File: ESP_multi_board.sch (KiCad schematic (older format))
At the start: 20 parts, among them P101 CONN_01X02, P102 CONN_01X06, P103 CONN_01X02, P104 CONN_01X06, P105 CONN_01X12, P106 CONN_01X03, P107 JUMPER1, P108 CONN_I2C_MPU6050, P109 CONN_01X03, P110 CONN_01X03, P111 CONN_DIGITAL, P112 CONN_I2C, U101 L293DD, U102 ESP-12, U103 MAX11605EEE+, U104 MCP23008

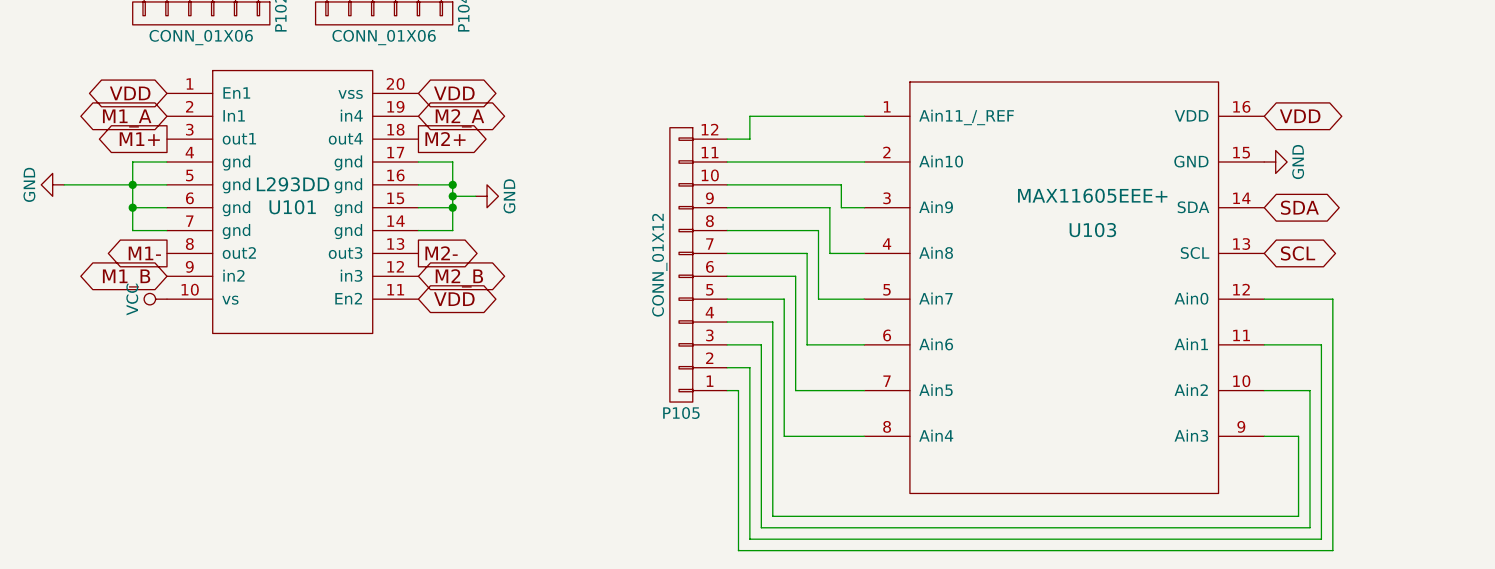
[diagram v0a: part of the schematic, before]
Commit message: pendiente de enrutar, TODO: incluir diodos baterias, meditar los jumpers
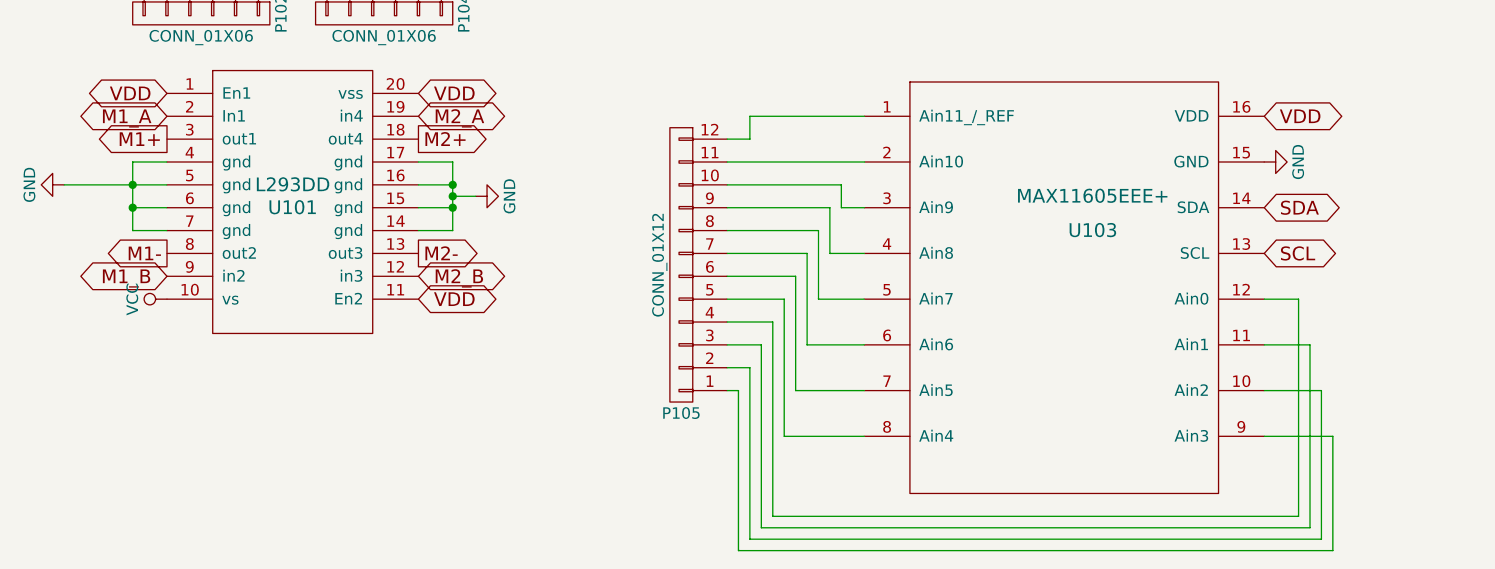
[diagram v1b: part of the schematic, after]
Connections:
- net at U103.10 (Ain2): now also P105.2 (P2); no longer P105.3 (P3)
- net at U103.11 (Ain1): now also P105.3 (P3); no longer P105.2 (P2)
- net at U103.12 (Ain0): now also P105.4 (P4); no longer P105.1 (P1)
- net at U103.9 (Ain3): now also P105.1 (P1); no longer P105.4 (P4)
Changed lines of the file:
@@
 	4050 6200 6350 6200
 Wire Wire Line
-	6350 6200 6350 5850
-Wire Wire Line
-	6350 5850 6200 5850
+	6350 6200 6350 5250
 Wire Wire Line
 	3850 5450 4000 5450
@@
 	4000 6250 6400 6250
 Wire Wire Line
-	6400 6250 6400 5650
-Wire Wire Line
-	6400 5650 6200 5650
+	6400 6250 6400 5450
 Wire Wire Line
 	3950 5550 3950 6300
@@
 	3950 6300 6450 6300
 Wire Wire Line
-	6450 6300 6450 5450
+	6450 6300 6450 5650
 Wire Wire Line
-	6450 5450 6200 5450
-Wire Wire Line
-	6200 5250 6500 5250
-Wire Wire Line
-	6500 5250 6500 6350
+	6500 5850 6500 6350
 Wire Wire Line
 	6500 6350 3900 6350
@@
 VDD
 Wire Wire Line
-	1400 4950 1250 4950
+	1250 4950 1400 4950
 Wire Wire Line
-	1250 4950 1250 4650
+	1250 4650 1250 4950
 Wire Wire Line
 	1250 4650 1400 4650
@@
 	1400 4850 1250 4850
 Connection ~ 1250 4850
+Wire Wire Line
+	6350 5250 6200 5250
+Wire Wire Line
+	6400 5450 6200 5450
+Wire Wire Line
+	6450 5650 6200 5650
+Wire Wire Line
+	6500 5850 6200 5850
 $EndSCHEMATC
